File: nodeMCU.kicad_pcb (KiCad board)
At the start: 2 copper layers, 27 x 50 mm, 41 parts, among them J1 USB_B_Micro, J2 Conn_01x15, J3 Conn_01x15, Q1 S8050, Q2 S8050, SW1 RESET, SW2 FLASH, U1 AP1117-33, U2 CP2102N-A01-GQFN28, U3 ESP-12E

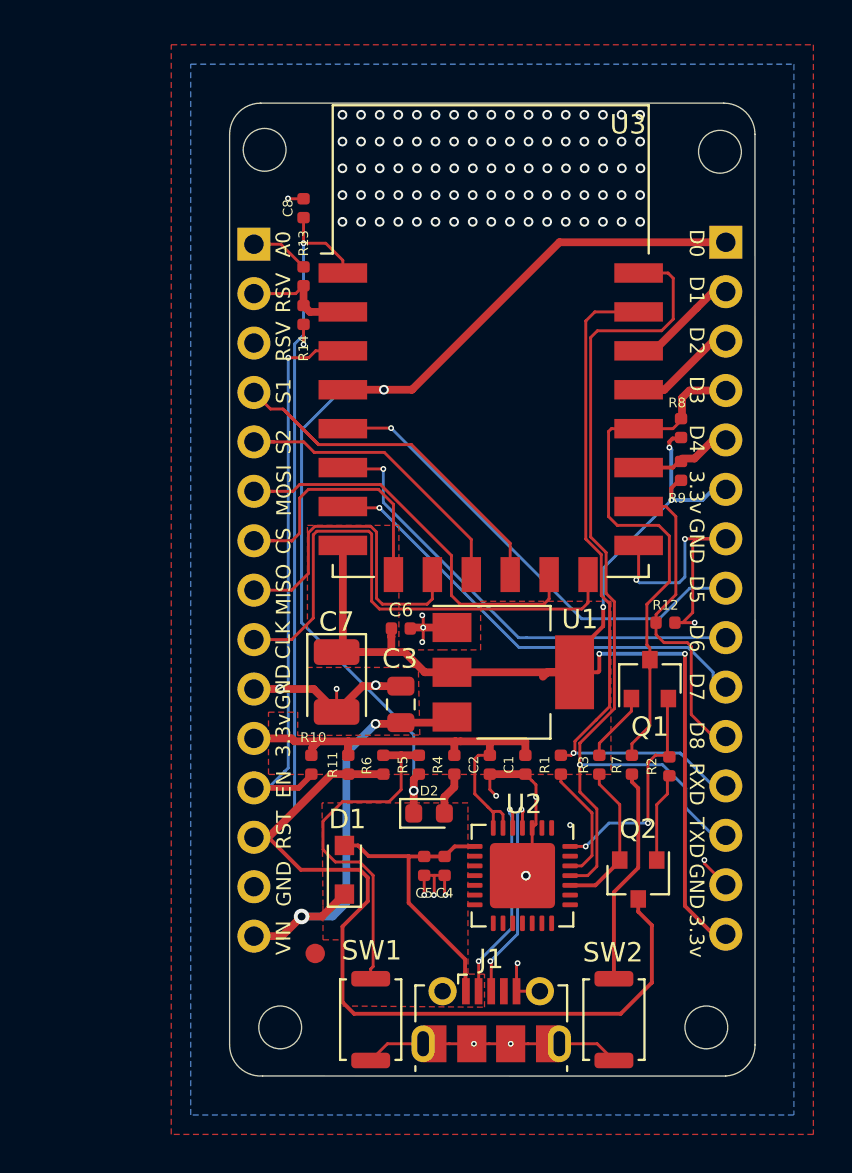
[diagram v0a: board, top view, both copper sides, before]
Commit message: Agrego comentarios del Docente
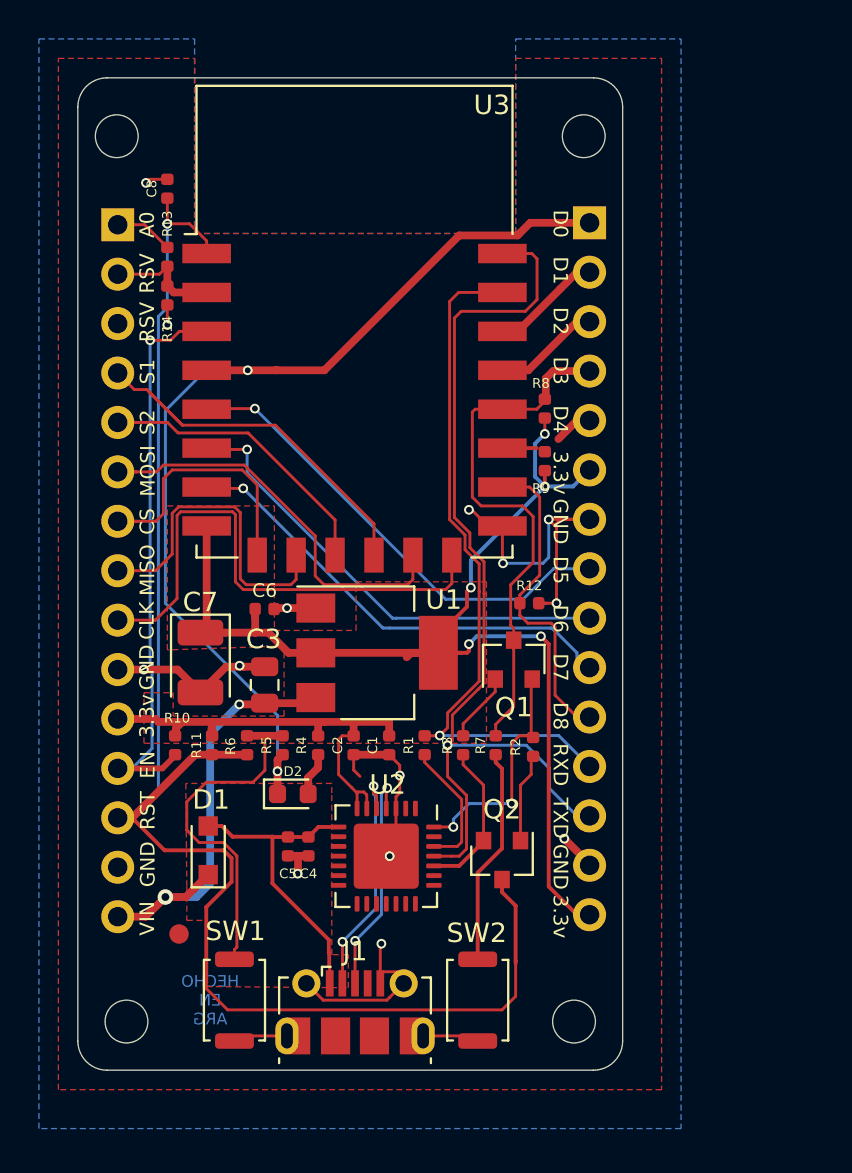
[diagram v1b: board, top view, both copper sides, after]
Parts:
- moved H2 7.91 mm to (127.5, 110.5)
- moved H4 7.63 mm to (127.0, 65.0)
- moved J2 7.07 mm to (127.0, 69.5)
- moved C1 7.07 mm to (141.0, 96.3)
- moved C2 7.07 mm to (139.2, 96.3)
- moved C3 7.07 mm to (134.6, 93.2)
- moved C4 7.07 mm to (136.8, 101.5)
- moved C5 7.07 mm to (135.8, 101.5)
- moved C6 7.07 mm to (134.6, 89.3)
- moved C7 7.07 mm to (131.3, 92.0)
- moved C8 7.07 mm to (129.6, 67.7)
- moved D1 7.07 mm to (131.7, 101.7)
- moved D2 7.07 mm to (136.1, 98.8)
- moved FID1 7.07 mm to (130.2, 106.0)
- moved J3 7.07 mm to (151.3, 69.5)
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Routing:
- net /nRST: track 77.2 -> 79.1 mm
- net /GPIO_2: track 4.42 -> 3.12 mm
- net Net-(J1-Pad2): track 11.1 -> 12.2 mm
- net VBUS: track 15.0 -> 15.9 mm
- net /RXD: track 35.0 -> 35.8 mm
- net /GPIO_16: track 50.3 -> 51.0 mm
- net +3V3: track 84.3 -> 85.0 mm
- net Net-(R3-Pad2): track 6.20 -> 6.80 mm
- net /TXD: track 47.9 -> 48.5 mm
- net GND: track 62.8 -> 62.3 mm, vias 107 -> 14
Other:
- board size 27 x 50 mm -> 28 x 51 mm
- rule via_min_size: 0.15 -> 0.5
- board text added: "Esta placa fue desarrollada en el marco de la materia “Diseño de circuitos impresos” pertenceciente a la Carrera de Especializacion en Sistemas Embebidos de la UBA. Para este proyecto se tomo como premisa usar los mismo tamaños que su original. Es por esto que algunos de los componentes poseen encapsulados de tamaño reducido. Grillas: 1mm, 0.5mm, 0.10mm Vias: 0.5/0.3mm Margen: 0.1mm Pistas: 0.4mm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"
- board text added: "HECHO EN ARG"
- board text removed: "Esta placa fue desarrollada en el marco de la materia "Diseño de circuitos impresos" pertenceciente a la Carrera de Especializacion en Sistemas Embebidos de la UBA. Para este proyecto se tomo como premisa usar los mismo tamaños que su original. Es por esto que algunos de los componentes poseen encapsulados de tamaño reducido. Grillas: 1mm, 0.5mm, 0.10mm Vias: 0.30/0.15mm, 0.5/0.3mm Margen: 0.2mm 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"
- board text removed: "HECHO EN ARGENTINA"
